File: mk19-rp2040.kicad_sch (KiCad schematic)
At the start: 134 parts, among them J1 USB_C_Receptacle_USB2.0, J10 Conn_01x02, J11 Conn_01x03_Socket, J12 USB_C_Receptacle_USB2.0, J13 USB_C_Receptacle_USB2.0, J2 Conn_01x03_Socket, J3 Conn_01x02_Socket, J4 Conn_01x06_Socket, J5 Conn_01x02, J7 Conn_01x02_Socket, J8 Conn_01x02_Socket, J9 Conn_01x02_Socket, T1 Conn_01x01_Socket, T10 Conn_01x01_Socket, T11 Conn_01x01_Socket, T12 Conn_01x01_Socket, T13 Conn_01x01_Socket, T14 Conn_01x01_Socket, T15 Conn_01x01_Socket, T2 Conn_01x01_Socket, T3 Conn_01x01_Socket, T5 Conn_01x01_Socket, T6 Conn_01x01_Socket, T7 Conn_01x01_Socket, T9 Conn_01x01_Socket, U1 RP2040, U10 1N4148W_C81598, U11 1N4148W_C81598, U12 1N4148W_C81598, U13 1N4148W_C81598, U14 1N4148W_C81598, U15 1N4148W_C81598, U2 USBLC6-2P6, U3 XC6210B332MR-G, U4 USBLC6-2P6, U5 W25Q128JVS, U6 8_01A0_008200, U7 8_01A0_008200, U8 USBLC6-2P6, U9 1N4148W_C81598, Y1 Crystal_GND24

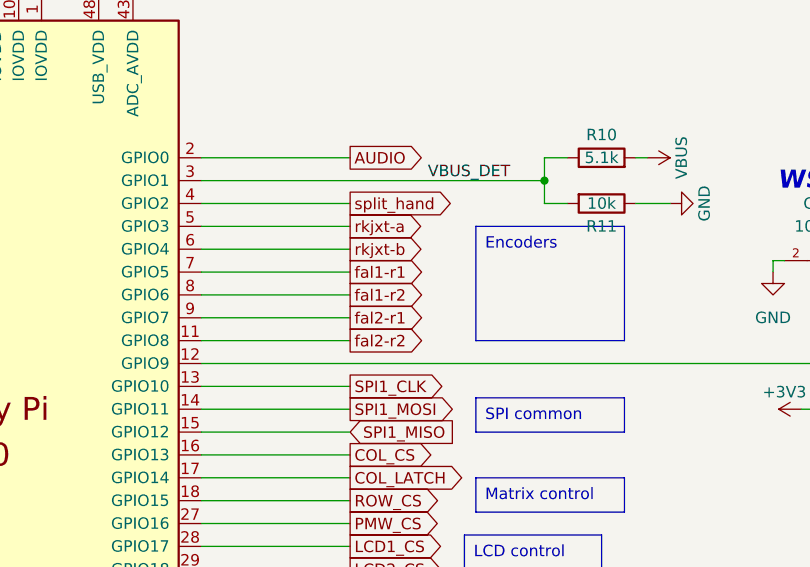
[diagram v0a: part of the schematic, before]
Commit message: even more progress, starting to come together.
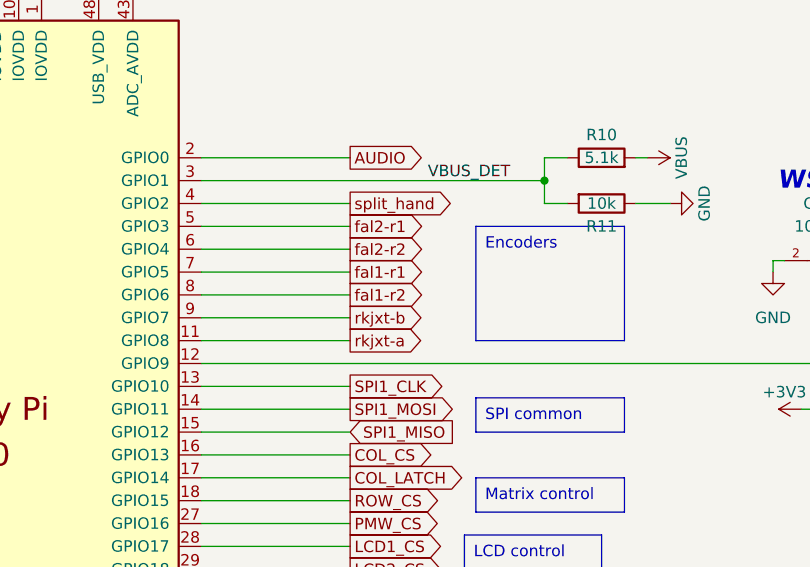
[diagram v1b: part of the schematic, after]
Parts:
- J10, J5: footprint drawings:PinHeader_1x02_P1.27mm_Vertical -> Connector_PinSocket_2.54mm:PinSocket_1x02_P2.54mm_Vertical
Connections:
- net fal2-r1: now also U1.5 (GPIO3); no longer U1.9 (GPIO7)
- net fal2-r2: now also U1.6 (GPIO4); no longer U1.11 (GPIO8)
- net rkjxt-a: now also U1.11 (GPIO8); no longer U1.5 (GPIO3)
- net rkjxt-b: now also U1.9 (GPIO7); no longer U1.6 (GPIO4)
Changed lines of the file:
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@@
 		)
 	)
-	(global_label "fal1-r1"
-		(shape output)
-		(at 504.19 77.47 0)
+	(global_label "row5"
+		(shape input)
+		(at 72.39 78.74 180)
 		(fields_autoplaced yes)
 		(effects
@@
 				(size 1.27 1.27)
 			)
-			(justify left)
+			(justify right)
 		)
 		(property "Intersheetrefs" "${INTERSHEET_REFS}"
-			(at 514.4927 77.47 0)
+			(at 64.9296 78.74 0)
 			(effects
 				(font
 					(size 1.27 1.27)
 				)
-				(justify left)
+				(justify right)
 				(hide yes)
 			)
 		)
 	)
-	(global_label "row5"
-		(shape input)
-		(at 72.39 78.74 180)
+	(global_label "col7"
+		(shape output)
+		(at 273.05 62.23 0)
 		(fields_autoplaced yes)
 		(effects
@@
 				(size 1.27 1.27)
 			)
-			(justify right)
+			(justify left)
 		)
 		(property "Intersheetrefs" "${INTERSHEET_REFS}"
-			(at 64.9296 78.74 0)
+			(at 280.1475 62.23 0)
 			(effects
 				(font
 					(size 1.27 1.27)
 				)
-				(justify right)
+				(justify left)
 				(hide yes)
 			)
 		)
 	)
-	(global_label "col7"
+	(global_label "fal2-r1"
 		(shape output)
-		(at 273.05 62.23 0)
+		(at 504.19 72.39 0)
 		(fields_autoplaced yes)
 		(effects
@@
 		)
 		(property "Intersheetrefs" "${INTERSHEET_REFS}"
-			(at 280.1475 62.23 0)
+			(at 514.4927 72.39 0)
 			(effects
 				(font
@@
 		)
 	)
-	(global_label "fal2-r2"
-		(shape output)
-		(at 504.19 85.09 0)
-		(fields_autoplaced yes)
-		(effects
-			(font
-				(size 1.27 1.27)
-			)
-			(justify left)
-		)
-		(property "Intersheetrefs" "${INTERSHEET_REFS}"
-			(at 514.4927 85.09 0)
-			(effects
-				(font
-					(size 1.27 1.27)
-				)
-				(justify left)
-				(hide yes)
-			)
-		)
-	)
 	(global_label "fal1-r2"
 		(shape input)
@@
 		)
 	)
-	(global_label "LED_MACRO_DI"
-		(shape input)
-		(at 247.65 69.85 180)
+	(global_label "fal1-r1"
+		(shape output)
+		(at 504.19 77.47 0)
 		(fields_autoplaced yes)
 		(effects
@@
 				(size 1.27 1.27)
 			)
-			(justify right)
+			(justify left)
 		)
 		(property "Intersheetrefs" "${INTERSHEET_REFS}"
-			(at 230.9972 69.85 0)
+			(at 514.4927 77.47 0)
 			(effects
 				(font
 					(size 1.27 1.27)
 				)
-				(justify right)
+				(justify left)
 				(hide yes)
 			)
 		)
 	)
-	(global_label "row1"
+	(global_label "LED_MACRO_DI"
 		(shape input)
-		(at 53.34 115.57 0)
+		(at 247.65 69.85 180)
 		(fields_autoplaced yes)
 		(effects
@@
 				(size 1.27 1.27)
 			)
-			(justify left)
+			(justify right)
 		)
 		(property "Intersheetrefs" "${INTERSHEET_REFS}"
-			(at 60.8004 115.57 0)
+			(at 230.9972 69.85 0)
 			(effects
 				(font
 					(size 1.27 1.27)
 				)
-				(justify left)
+				(justify right)
 				(hide yes)
 			)
 		)
 	)
-	(global_label "rkjxt-a"
-		(shape output)
-		(at 504.19 72.39 0)
+	(global_label "row1"
+		(shape input)
+		(at 53.34 115.57 0)
 		(fields_autoplaced yes)
 		(effects
@@
 		)
 		(property "Intersheetrefs" "${INTERSHEET_REFS}"
-			(at 514.0695 72.39 0)
+			(at 60.8004 115.57 0)
 			(effects
 				(font
@@
 		)
 	)
+	(global_label "fal2-r2"
+		(shape output)
+		(at 504.19 74.93 0)
+		(fields_autoplaced yes)
+		(effects
+			(font
+				(size 1.27 1.27)
+			)
+			(justify left)
+		)
+		(property "Intersheetrefs" "${INTERSHEET_REFS}"
+			(at 514.4927 74.93 0)
+			(effects
+				(font
+					(size 1.27 1.27)
+				)
+				(justify left)
+				(hide yes)
+			)
+		)
+	)
 	(global_label "row8"
 		(shape input)
@@
 		)
 	)
-	(global_label "fal1-r2"
-		(shape output)
-		(at 504.19 80.01 0)
-		(fields_autoplaced yes)
-		(effects
-			(font
-				(size 1.27 1.27)
-			)
-			(justify left)
-		)
-		(property "Intersheetrefs" "${INTERSHEET_REFS}"
-			(at 514.4927 80.01 0)
-			(effects
-				(font
-					(size 1.27 1.27)
-				)
-				(justify left)
-				(hide yes)
-			)
-		)
-	)
 	(global_label "row0"
 		(shape output)
@@
 		)
 	)
-	(global_label "rkjxt-b"
-		(shape output)
-		(at 504.19 74.93 0)
-		(fields_autoplaced yes)
-		(effects
-			(font
-				(size 1.27 1.27)
-			)
-			(justify left)
-		)
-		(property "Intersheetrefs" "${INTERSHEET_REFS}"
-			(at 514.0695 74.93 0)
-			(effects
-				(font
-					(size 1.27 1.27)
-				)
-				(justify left)
-				(hide yes)
-			)
-		)
-	)
 	(global_label "col1"
 		(shape output)
@@
 		)
 	)
-	(global_label "fal2-r1"
-		(shape output)
-		(at 504.19 82.55 0)
-		(fields_autoplaced yes)
-		(effects
-			(font
-				(size 1.27 1.27)
-			)
-			(justify left)
-		)
-		(property "Intersheetrefs" "${INTERSHEET_REFS}"
-			(at 514.4927 82.55 0)
-			(effects
-				(font
-					(size 1.27 1.27)
-				)
-				(justify left)
-				(hide yes)
-			)
-		)
-	)
 	(global_label "SPI1_CLK"
 		(shape input)
@@
 		)
 	)
+	(global_label "rkjxt-b"
+		(shape output)
+		(at 504.19 82.55 0)
+		(fields_autoplaced yes)
+		(effects
+			(font
+				(size 1.27 1.27)
+			)
+			(justify left)
+		)
+		(property "Intersheetrefs" "${INTERSHEET_REFS}"
+			(at 514.0695 82.55 0)
+			(effects
+				(font
+					(size 1.27 1.27)
+				)
+				(justify left)
+				(hide yes)
+			)
+		)
+	)
 	(global_label "col4"
 		(shape output)
@@
 		)
 	)
+	(global_label "fal1-r2"
+		(shape output)
+		(at 504.19 80.01 0)
+		(fields_autoplaced yes)
+		(effects
+			(font
+				(size 1.27 1.27)
+			)
+			(justify left)
+		)
+		(property "Intersheetrefs" "${INTERSHEET_REFS}"
+			(at 514.4927 80.01 0)
+			(effects
+				(font
+					(size 1.27 1.27)
+				)
+				(justify left)
+				(hide yes)
+			)
+		)
+	)
 	(global_label "row5"
 		(shape input)
@@
 		)
 	)
+	(global_label "rkjxt-a"
+		(shape output)
+		(at 504.19 85.09 0)
+		(fields_autoplaced yes)
+		(effects
+			(font
+				(size 1.27 1.27)
+			)
+			(justify left)
+		)
+		(property "Intersheetrefs" "${INTERSHEET_REFS}"
+			(at 514.0695 85.09 0)
+			(effects
+				(font
+					(size 1.27 1.27)
+				)
+				(justify left)
+				(hide yes)
+			)
+		)
+	)
 	(global_label "row11"
 		(shape output)
@@
 			)
 		)
-		(property "Footprint" "drawings:PinHeader_1x02_P1.27mm_Vertical"
+		(property "Footprint" "Connector_PinSocket_2.54mm:PinSocket_1x02_P2.54mm_Vertical"
 			(at 354.33 189.23 0)
 			(effects
@@
 			)
 		)
-		(property "Footprint" "drawings:PinHeader_1x02_P1.27mm_Vertical"
+		(property "Footprint" "Connector_PinSocket_2.54mm:PinSocket_1x02_P2.54mm_Vertical"
 			(at 410.21 123.19 0)
 			(effects
